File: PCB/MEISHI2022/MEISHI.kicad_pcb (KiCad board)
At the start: 2 copper layers, 91 x 55 mm, 37 parts, among them IC1 TB67H450FNG,EL, IC2 TB67H450FNG,EL, J1 AC CONNECTOR OUT, J10 Motor0, J11 Motor1, J2 USB_B_Micro, J3 AC CONNECTOR IN, J4 Conn_01x04, J5 IO0, J6 IO2, J7 IO1, J9 Motor Power, K1 942H-2C-5DS, SW1 SW_MEC_5E, SW2 SW_MEC_5E, U1 AZ1117-3.3, U2 TLP172AM, U3 ESP32-WROOM-32D

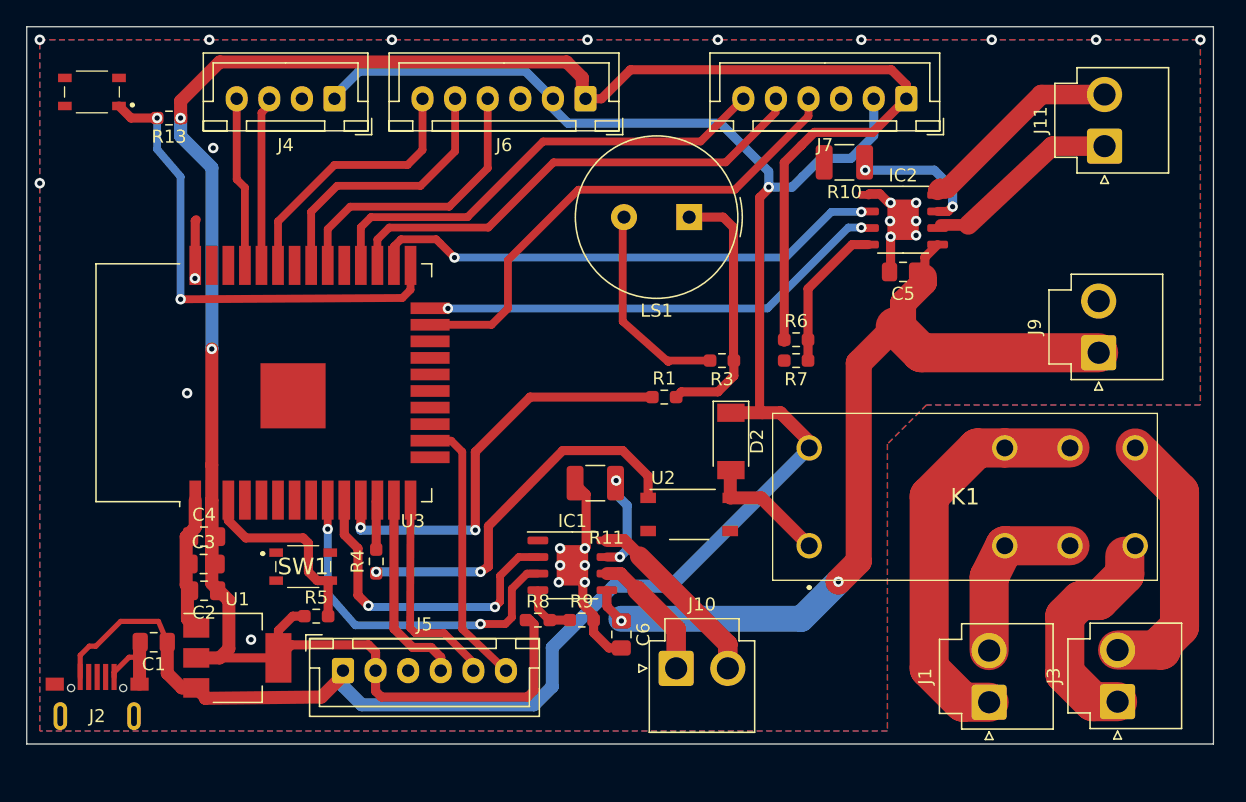
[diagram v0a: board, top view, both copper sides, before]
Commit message: feat MEISHI
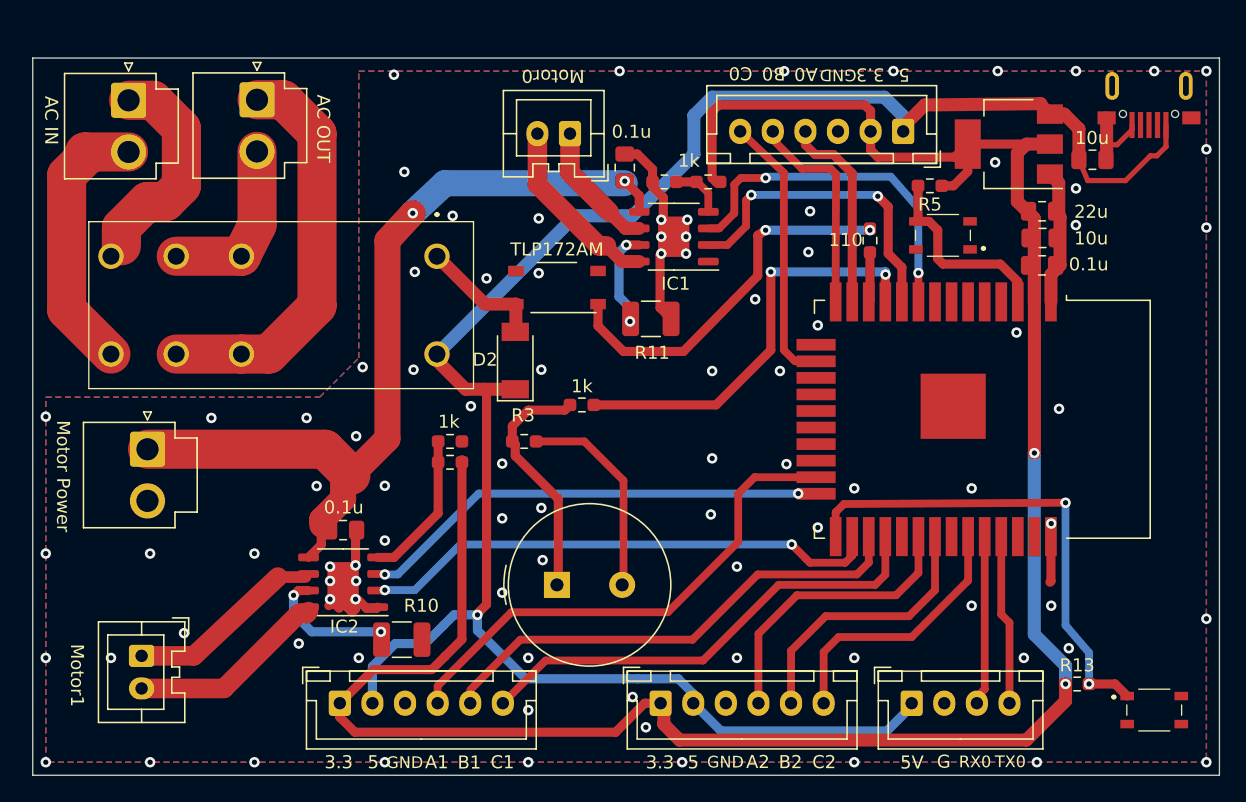
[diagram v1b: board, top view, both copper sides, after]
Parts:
- J10, J11: footprint Connector_JST:JST_VH_B2P-VH_1x02_P3.96mm_Vertical -> Connector_JST:JST_XA_B02B-XASK-1_1x02_P2.50mm_Vertical
- moved SW2 94.2 mm to (106.5, 72.4), turned to 0 degrees
- moved J2 94.0 mm to (106.1, 24.5), turned to 180 degrees
- moved J3 88.8 mm to (27.8, 25.6), turned to -90 degrees
- moved J11 83.5 mm to (28.8, 68.2), turned to -90 degrees
- moved R13 82.1 mm to (100.5, 70.4), turned to 0 degrees
- moved C1 80.9 mm to (101.7, 30.2), turned to 0 degrees
- moved J9 73.3 mm to (29.3, 52.4), turned to -90 degrees
- moved J1 72.7 mm to (37.7, 25.6), turned to -90 degrees
- moved U1 71.1 mm to (95.3, 29.0), turned to 180 degrees
- moved C2 70.5 mm to (97.9, 34.1), turned to 0 degrees
- moved C3 69.0 mm to (97.9, 36.2), turned to 180 degrees
- moved C4 67.5 mm to (97.9, 38.3), turned to 180 degrees
- moved J4 64.1 mm to (87.9, 71.9), turned to 0 degrees
- moved J7 63.5 mm to (44.0, 71.9), turned to 0 degrees
- moved J5 59.6 mm to (87.2, 28.0), turned to 180 degrees
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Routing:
- net GND: track 52.4 -> 56.7 mm, vias 25 -> 91
- net Net-(LS1-Pad1): track 20.2 -> 18.8 mm
- net /DRIVER1_OUT2: track 15.8 -> 15.2 mm
- net (no net): vias 1 -> 0
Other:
- board text added: "3.3"
- board text added: "5"
- board text added: "5V"
- board text added: "A0"
- board text added: "A1"
- board text added: "A2"
- board text added: "AC 100V"
- board text added: "AC IN"
- board text added: "AC OUT"
- board text added: "B0"
- board text added: "B1"
- board text added: "B2"
- board text added: "C0"
- board text added: "C1"
- board text added: "C2"
- board text added: "DANGER ZONE"
- board text added: "G"
- board text added: "GND"
- board text added: "HIGH VOLTAGE"
- board text added: "Motor Power"
- board text added: "Motor0"
- board text added: "Motor1"
- board text added: "RX0"
- board text added: "TX0"
